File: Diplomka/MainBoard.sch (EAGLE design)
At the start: 44 parts, among them K1 ARK550/2, Q1 PT15-21C/TR8, Q2 BC817-40LT1SMD, Q3 SS8050-G, Q4 SS8050-G, U1 ESP32-WROOM-32, U2 AMS1117-3.3

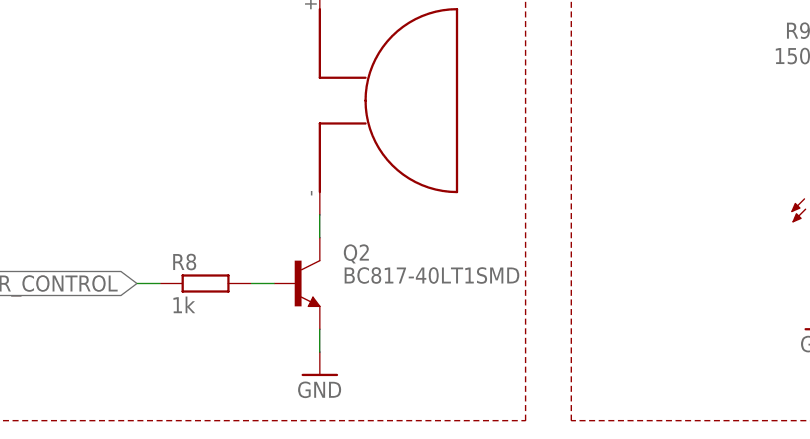
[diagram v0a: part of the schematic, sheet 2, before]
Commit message: Udělána objednávka.
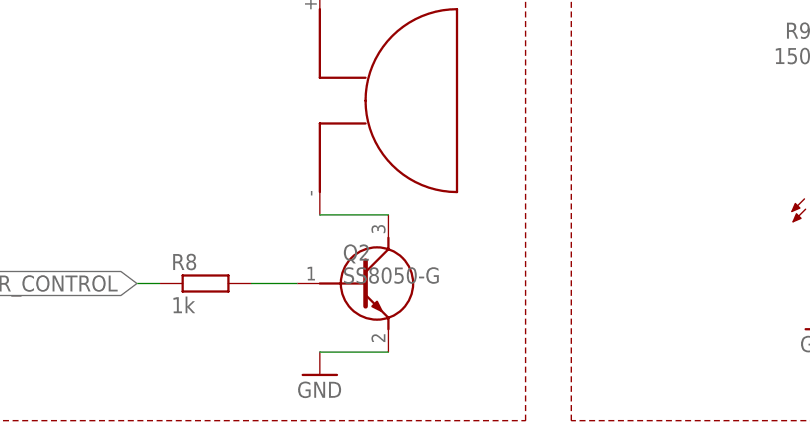
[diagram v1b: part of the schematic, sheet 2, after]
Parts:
- Q2: value BC817-40LT1SMD -> SS8050-G; device transistor-npn:BC817-40LT1SMD -> SS8050-G:SS8050-G
- R16, R17: value (none) -> 10k
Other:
- moved on the sheet: Q2
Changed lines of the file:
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@@
 <part name="U$3" library="myParts" deviceset="GY4466" device=""/>
 <part name="U$4" library="myParts" deviceset="BUZZER" device=""/>
-<part name="Q2" library="transistor-npn" library_urn="urn:adsk.eagle:library:398" deviceset="BC817*" device="SMD" package3d_urn="urn:adsk.eagle:package:28748/2" technology="-40LT1"/>
+<part name="Q2" library="SS8050-G" deviceset="SS8050-G" device=""/>
 <part name="GND6" library="supply1" library_urn="urn:adsk.eagle:library:371" deviceset="GND" device=""/>
 <part name="R8" library="rcl" library_urn="urn:adsk.eagle:library:334" deviceset="R-EU_" device="R0805" package3d_urn="urn:adsk.eagle:package:23553/2" value="1k"/>
@@
 <part name="Q3" library="SS8050-G" deviceset="SS8050-G" device=""/>
 <part name="Q4" library="SS8050-G" deviceset="SS8050-G" device=""/>
-<part name="R16" library="rcl" library_urn="urn:adsk.eagle:library:334" deviceset="R-EU_" device="R0805" package3d_urn="urn:adsk.eagle:package:23553/2"/>
-<part name="R17" library="rcl" library_urn="urn:adsk.eagle:library:334" deviceset="R-EU_" device="R0805" package3d_urn="urn:adsk.eagle:package:23553/2"/>
+<part name="R16" library="rcl" library_urn="urn:adsk.eagle:library:334" deviceset="R-EU_" device="R0805" package3d_urn="urn:adsk.eagle:package:23553/2" value="10k"/>
+<part name="R17" library="rcl" library_urn="urn:adsk.eagle:library:334" deviceset="R-EU_" device="R0805" package3d_urn="urn:adsk.eagle:package:23553/2" value="10k"/>
 </parts>
 <sheets>
@@
 <segment>
 <pinref part="Q2" gate="G$1" pin="E"/>
-<wire x1="142.24" y1="20.32" x2="142.24" y2="17.78" width="0.1524" layer="91"/>
+<wire x1="149.86" y1="17.78" x2="142.24" y2="17.78" width="0.1524" layer="91"/>
 <pinref part="GND6" gate="1" pin="GND"/>
 </segment>
@@
 <pinref part="Q2" gate="G$1" pin="C"/>
 <pinref part="U$4" gate="G$1" pin="-"/>
-<wire x1="142.24" y1="30.48" x2="142.24" y2="33.02" width="0.1524" layer="91"/>
+<wire x1="149.86" y1="33.02" x2="142.24" y2="33.02" width="0.1524" layer="91"/>
 </segment>
 </net>
@@
 <pinref part="R8" gate="G$1" pin="2"/>
 <pinref part="Q2" gate="G$1" pin="B"/>
-<wire x1="134.62" y1="25.4" x2="137.16" y2="25.4" width="0.1524" layer="91"/>
-</segment>
-</net>
+<wire x1="134.62" y1="25.4" x2="139.7" y2="25.4" width="0.1524" layer="91"/>
+</segment>
+</net>
